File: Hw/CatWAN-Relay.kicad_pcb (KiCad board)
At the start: 2 copper layers, 50 x 86.9 mm, 86 parts, among them J2 INPUTS, J3 OUTPUTS, J4 I2C, J5 Serial, P1 USB_C_Plug_USB2.0, Q1 MMBT2222A, Q2 MMBT2222A, Q3 MMBT2222A, SW1 BOOT, SW2 RESET, U1 AT3H7C-CuH-S, U2 RFM95W-915-868, U3 AT3H7C-CuH-S, U4 AT3H7C-CuH-S, U6 LM2596_DC-DC, U7 AP2114H-3.3TRG1, U8 ESP32-C6-WROOM-1U-N4, Y1 UD2-3NU, Y2 UD2-3NU, Y3 UD2-3NU

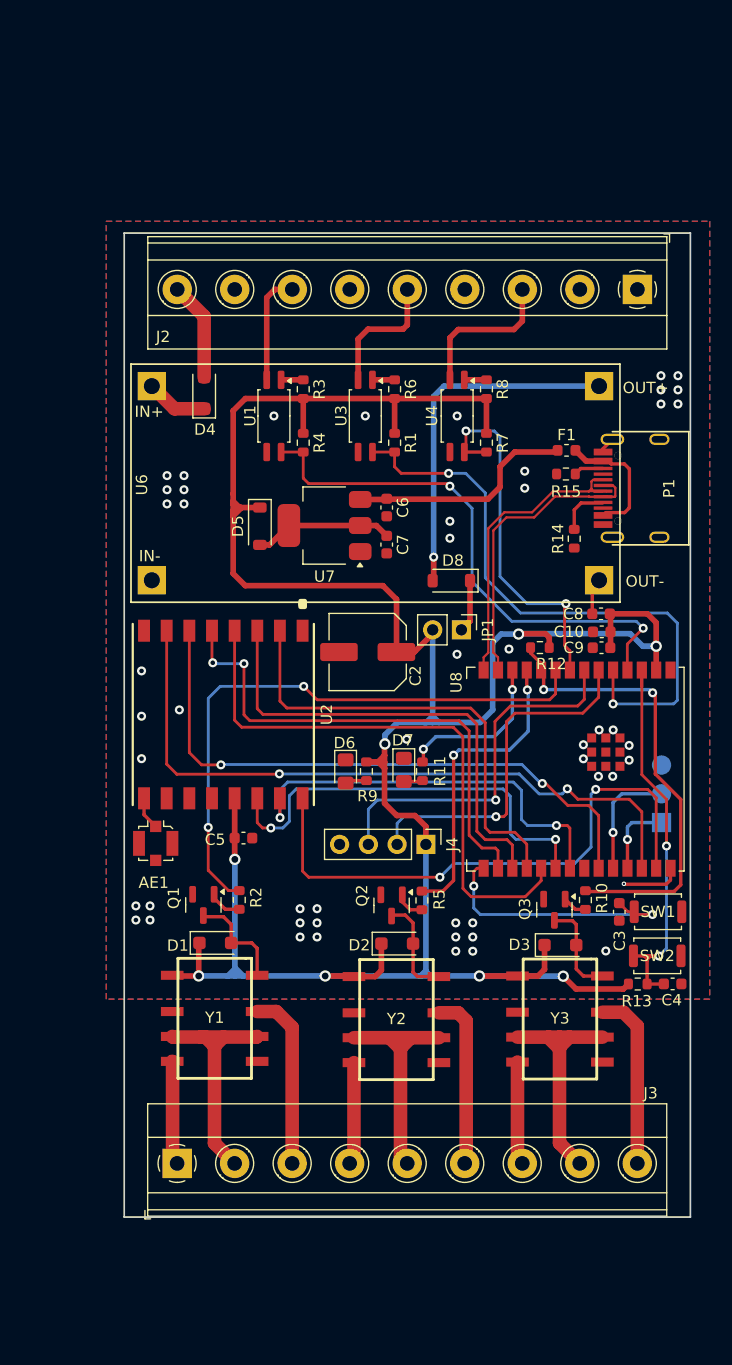
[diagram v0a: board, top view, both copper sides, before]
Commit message: feat: files_modified, _pro, _pcb & _sch
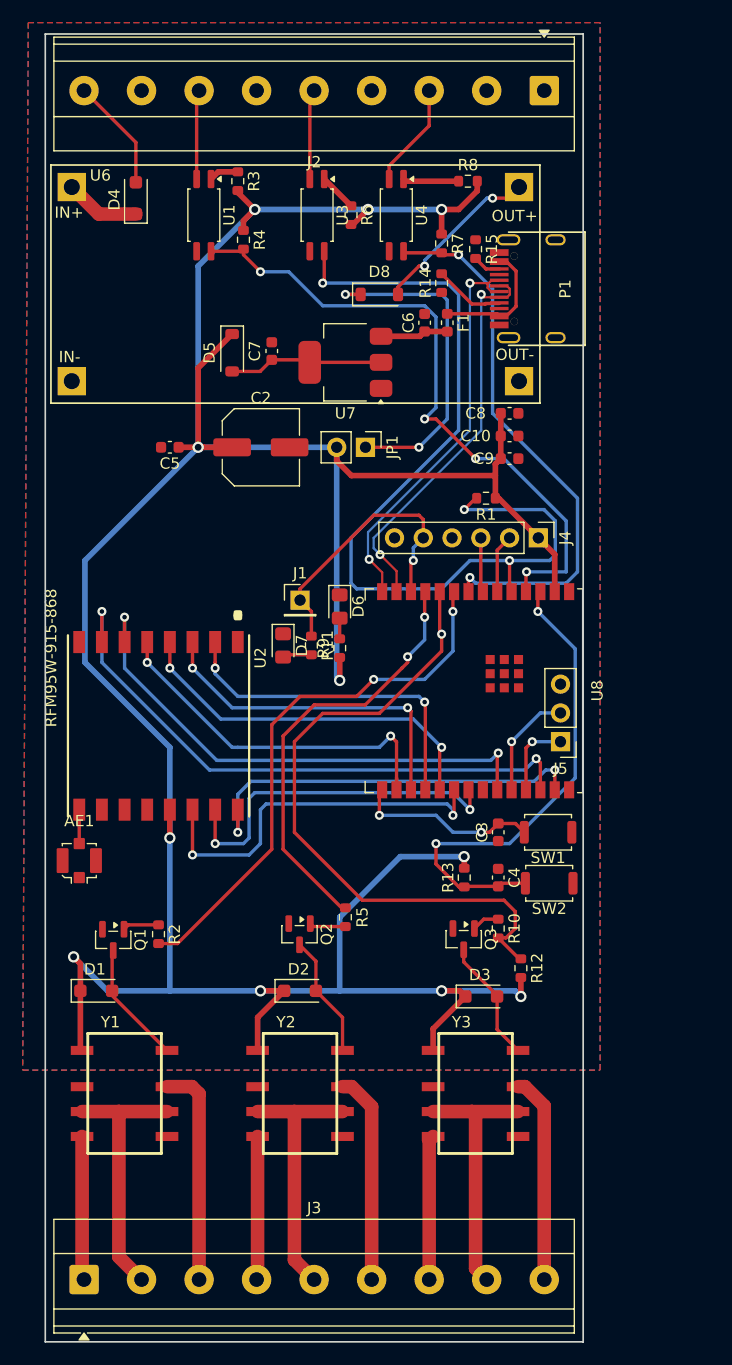
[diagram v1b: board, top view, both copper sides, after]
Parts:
- removed G***: LOGO, agroin:electronic_cats_logo_8x6
- removed kibuzzard-67649598: G***, kibuzzard-67649598
- removed kibuzzard-676495AB: G***, kibuzzard-676495AB
- removed kibuzzard-676D7180: G***, kibuzzard-676D7180
- removed kibuzzard-676D7534: G***, kibuzzard-676D7534
- removed kibuzzard-676D753C: G***, kibuzzard-676D753C
- removed kibuzzard-676D7543: G***, kibuzzard-676D7543
- removed kibuzzard-676D7549: G***, kibuzzard-676D7549
- removed kibuzzard-676D7550: G***, kibuzzard-676D7550
- removed kibuzzard-676D7558: G***, kibuzzard-676D7558
- removed kibuzzard-676D7562: G***, kibuzzard-676D7562
- removed kibuzzard-676D7567: G***, kibuzzard-676D7567
- removed kibuzzard-676D757C: G***, kibuzzard-676D757C
- removed kibuzzard-676D7581: G***, kibuzzard-676D7581
- removed kibuzzard-676D758E: G***, kibuzzard-676D758E
- removed kibuzzard-676D75AF: G***, kibuzzard-676D75AF
- removed kibuzzard-676D75BA: G***, kibuzzard-676D75BA
- removed kibuzzard-676D829F: G***, kibuzzard-676D829F
- removed kibuzzard-676D82E6: G***, kibuzzard-676D82E6
- removed kibuzzard-676D82FB: G***, kibuzzard-676D82FB
- removed kibuzzard-676D8308: G***, kibuzzard-676D8308
- removed kibuzzard-676D8313: G***, kibuzzard-676D8313
- removed kibuzzard-676D831D: G***, kibuzzard-676D831D
- removed kibuzzard-676D8326: G***, kibuzzard-676D8326
- removed kibuzzard-676D832F: G***, kibuzzard-676D832F
- removed kibuzzard-676D8337: G***, kibuzzard-676D8337
- removed kibuzzard-676D833E: G***, kibuzzard-676D833E
- removed kibuzzard-677EAF7D: G***, kibuzzard-677EAF7D
- removed kibuzzard-677EAF9B: G***, kibuzzard-677EAF9B
- removed kibuzzard-677EAFAE: G***, kibuzzard-677EAFAE
- removed kibuzzard-677EAFBC: G***, kibuzzard-677EAFBC
- added J1: Conn_01x01, Connector_PinHeader_2.54mm:PinHeader_1x01_P2.54mm_Vertical, F.Cu at (57.0, 70.0)
- D7: value Rx -> SS0_LED
- J4: footprint Connector_PinHeader_2.54mm:PinHeader_1x04_P2.54mm_Vertical -> Connector_PinHeader_2.54mm:PinHeader_1x06_P2.54mm_Vertical
- J5: moved to F.Cu
- U8: footprint PCM_Espressif:ESP32-C6-WROOM-1U -> Espressif:ESP32-C6-WROOM-1U
- moved C5 35.1 mm to (45.5, 56.5), turned to 180 degrees
- moved J4 28.8 mm to (78.0, 64.5)
- moved R12 28.4 mm to (76.5, 102.5), turned to -90 degrees
- moved D8 26.1 mm to (64.0, 43.0), turned to 0 degrees
- moved R14 25.4 mm to (69.5, 42.0)
- moved R15 21.4 mm to (72.5, 39.0), turned to -90 degrees
- moved C2 20.4 mm to (53.5, 56.5), turned to 0 degrees
- moved C7 19.9 mm to (54.5, 48.0), turned to 90 degrees
- moved P1 19.9 mm to (75.4, 42.5)
- moved C8 19.5 mm to (75.5, 53.5), turned to 0 degrees
- moved J2 19.4 mm to (78.6, 25.0)
- moved R3 19.3 mm to (51.5, 33.0)
- moved C10 19.1 mm to (75.5, 55.5), turned to 0 degrees
- moved U6 19.0 mm to (35.0, 31.6)
- moved U1 18.8 mm to (48.5, 36.0)
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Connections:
- net /SS renamed /SS0
- J4 pad 4: GND -> /<NO NET>
- R11 pad 1: /RX_LED -> /SS1
- U8 pad 12: /RX_LED -> /SS1
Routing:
- net +3V3: track 237.5 -> 285.1 mm, vias 8 -> 11
- net /SCL: track 33.0 -> 4.82 mm, vias 1 -> 0
- net /DI2: track 53.9 -> 80.3 mm, vias 2 -> 3
- net /SDA: track 31.5 -> 5.20 mm, vias 1 -> 0
- net /SS1: track 0.00 -> 25.1 mm, vias 0 -> 1
- net Net-(D8-K): track 4.65 -> 29.3 mm, vias 0 -> 2
- net /SCK: track 51.0 -> 33.0 mm, vias 0 -> 2
- net /DO1: track 40.6 -> 58.1 mm, vias 2 -> 1
- net /DI1: track 32.4 -> 48.8 mm
- net Net-(D8-A): track 31.3 -> 15.3 mm, vias 1 -> 2
- net /RX_LED: track 14.4 -> 0.00 mm, vias 2 -> 0
- net /DIO2: track 50.4 -> 36.0 mm
- net VBUS: track 20.3 -> 6.03 mm
- net /MOSI: track 42.0 -> 30.1 mm, vias 0 -> 2
- net /SS0: track 44.6 -> 32.9 mm
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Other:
- board size 50 x 86.9 mm -> 47.5 x 115.5 mm
